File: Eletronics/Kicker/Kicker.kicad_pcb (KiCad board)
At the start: 2 copper layers, 37.9 x 20.5 mm, 12 parts, among them J1 Solenoid, J2 Signal, J3 Battery, Q1 IRF540N

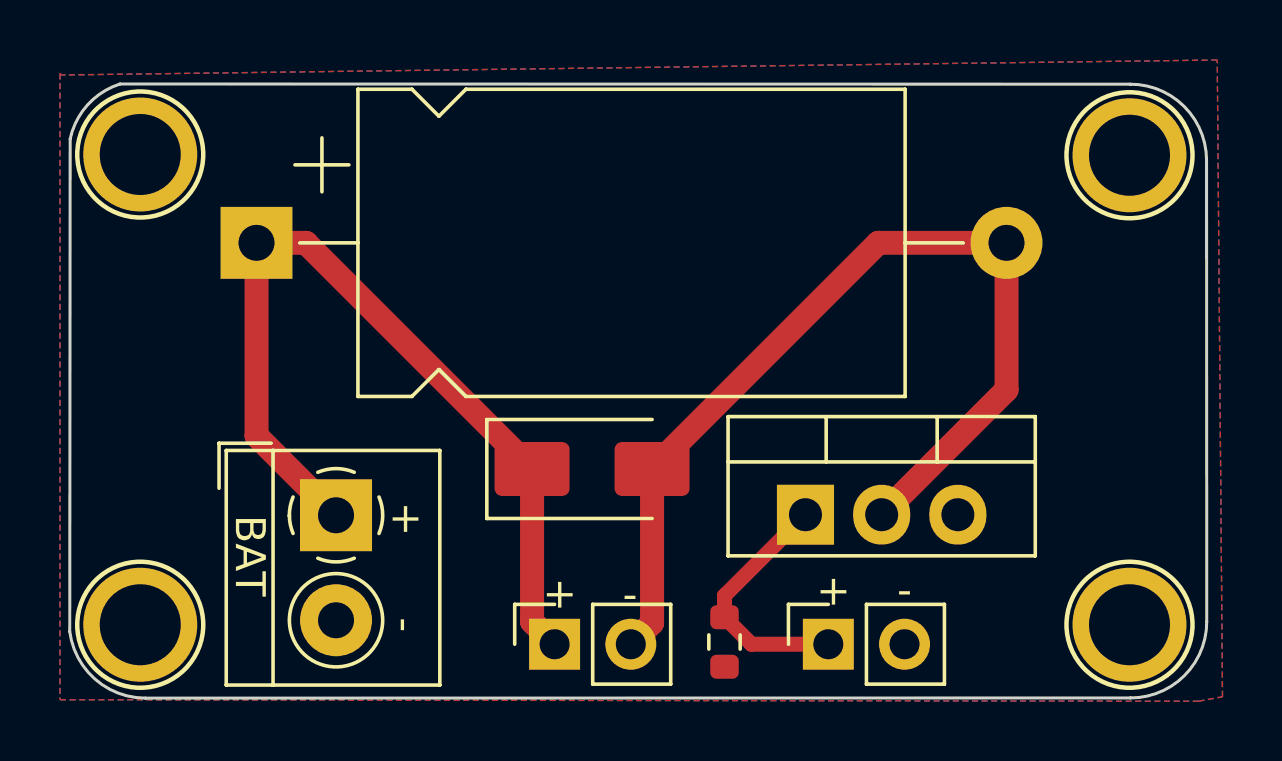
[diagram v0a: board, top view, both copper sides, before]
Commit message: Kicker modified
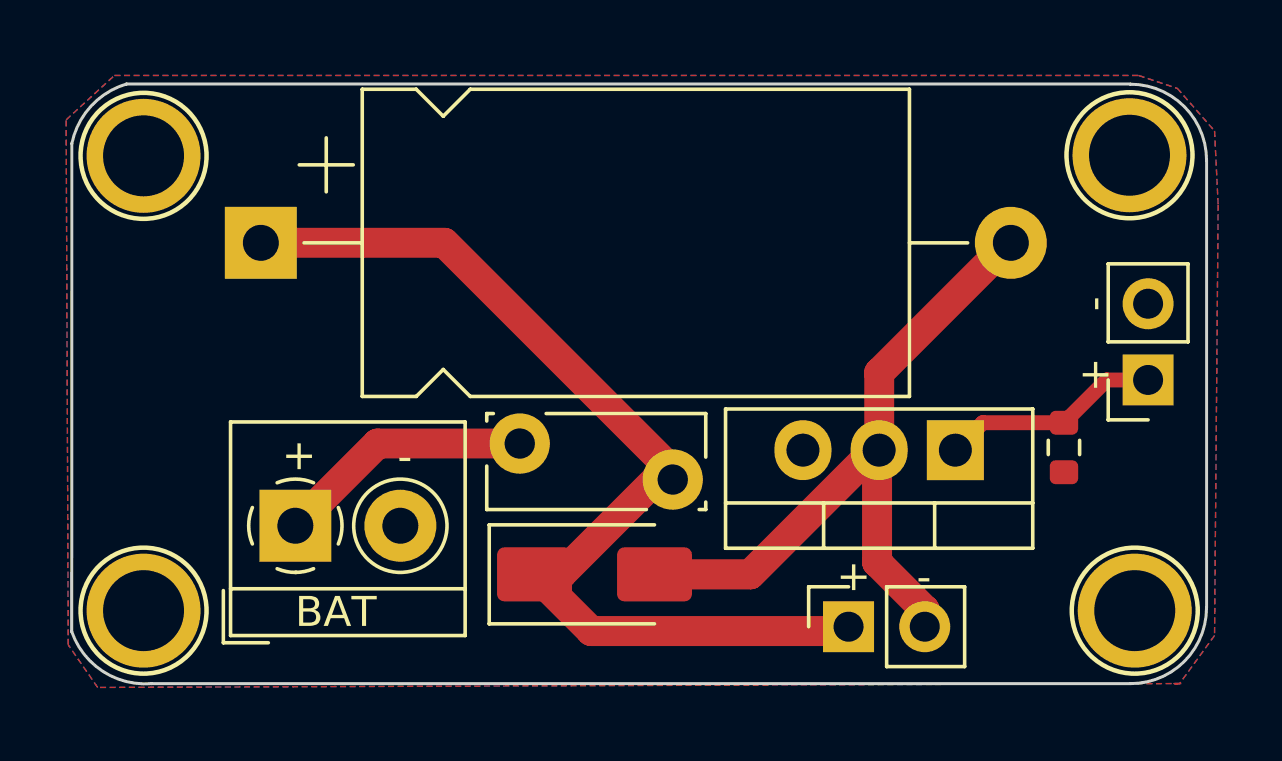
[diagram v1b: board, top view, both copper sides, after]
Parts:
- added F2: Fuse_Polarized, Fuse:Fuse_Bourns_MF-RG300, F.Cu at (131.7, 63.2)
- moved J2 13.8 mm to (152.6, 61.0), turned to 180 degrees
- moved R1 13.0 mm to (149.8, 63.3)
- moved J1 9.82 mm to (142.7, 69.3)
- moved Q1 5.44 mm to (146.2, 63.4), turned to 180 degrees
- moved D1 3.51 mm to (134.2, 67.5)
- moved G 3.33 mm to (141.2, 56.8)
- moved J3 1.40 mm to (124.2, 65.9), turned to 0 degrees
- moved H4 0.50 mm to (152.2, 68.7)
- moved H4 0.48 mm to (119.2, 68.7)
- moved C1 0.14 mm to (123.1, 56.5)
- moved H4 0.12 mm to (119.2, 53.6)
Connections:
- C1 pad 1: +BATT -> Net-(D1-K)
- D1 pad 1: +BATT -> Net-(D1-K)
- J1 pad 1: +BATT -> Net-(D1-K)
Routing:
- net Net-(D1-K): track 0.00 -> 34.4 mm
- net +BATT: track 28.6 -> 8.61 mm
- net Net-(D1-A): track 31.9 -> 24.5 mm
- net Net-(J2-Pin_1): track 8.37 -> 7.39 mm
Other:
- board size 37.9 x 20.5 mm -> 37.8 x 20 mm
